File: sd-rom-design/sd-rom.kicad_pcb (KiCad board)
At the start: 2 copper layers, 157.8 x 100 mm, 12 parts, among them J1 JAE50, J2 Conn_01x40, J3 Conn_01x40, J4 SD44, J5 Conn_01x04_Male, U1 ATtiny13A-SSU, U2 AMS1117-3.3

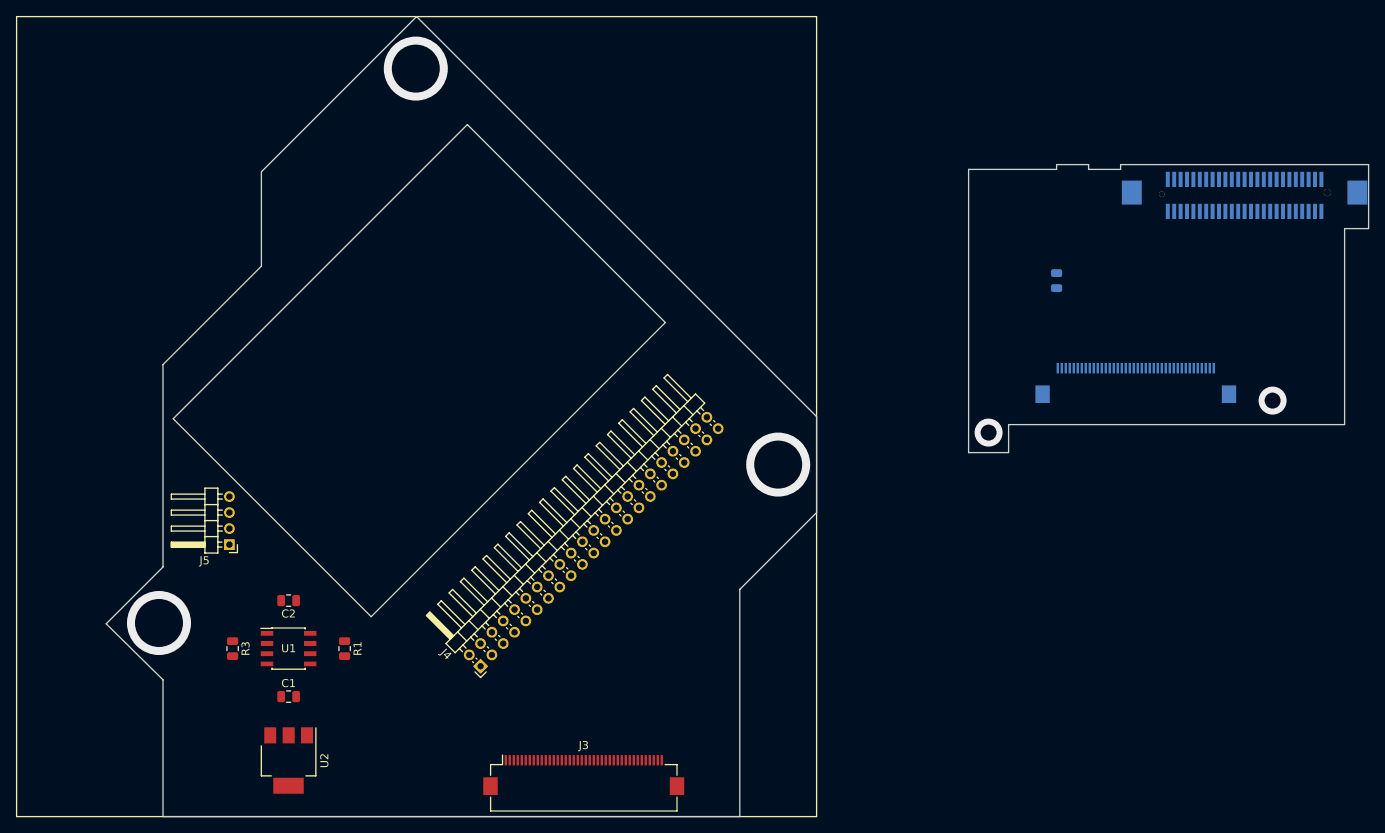
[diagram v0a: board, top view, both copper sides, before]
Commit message: board variant 3
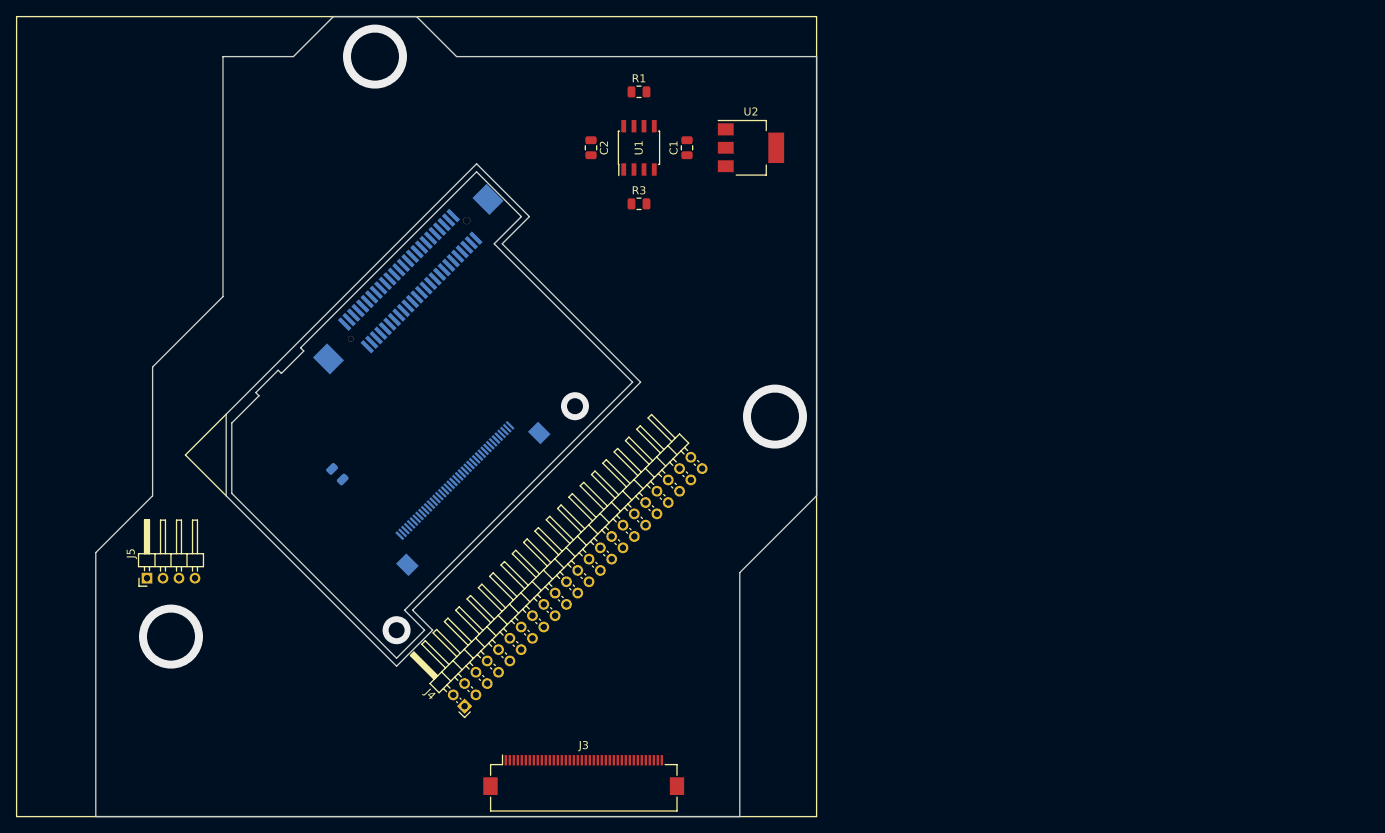
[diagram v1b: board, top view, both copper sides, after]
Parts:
- moved J1 105.1 mm to (39.8, 38.3), turned to 225 degrees
- moved U2 96.0 mm to (91.8, 16.4), turned to 0 degrees
- moved R2 93.1 mm to (40.1, 57.2), turned to 135 degrees
- moved J2 84.9 mm to (56.1, 59.3), turned to 225 degrees
- moved C1 84.8 mm to (83.8, 16.4), turned to 90 degrees
- moved R1 78.7 mm to (77.8, 9.40), turned to 0 degrees
- moved U1 76.4 mm to (77.8, 16.4), turned to 90 degrees
- moved R3 75.3 mm to (77.8, 23.4), turned to 0 degrees
- moved C2 68.1 mm to (71.8, 16.4), turned to 270 degrees
- moved J5 11.1 mm to (16.3, 70.2), turned to 90 degrees
- moved J4 5.39 mm to (56.0, 86.2)
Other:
- board size 157.8 x 100 mm -> 90.1 x 100 mm
